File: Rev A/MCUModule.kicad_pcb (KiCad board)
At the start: 2 copper layers, 1 part, among them U1 RaspberryPi_Pico

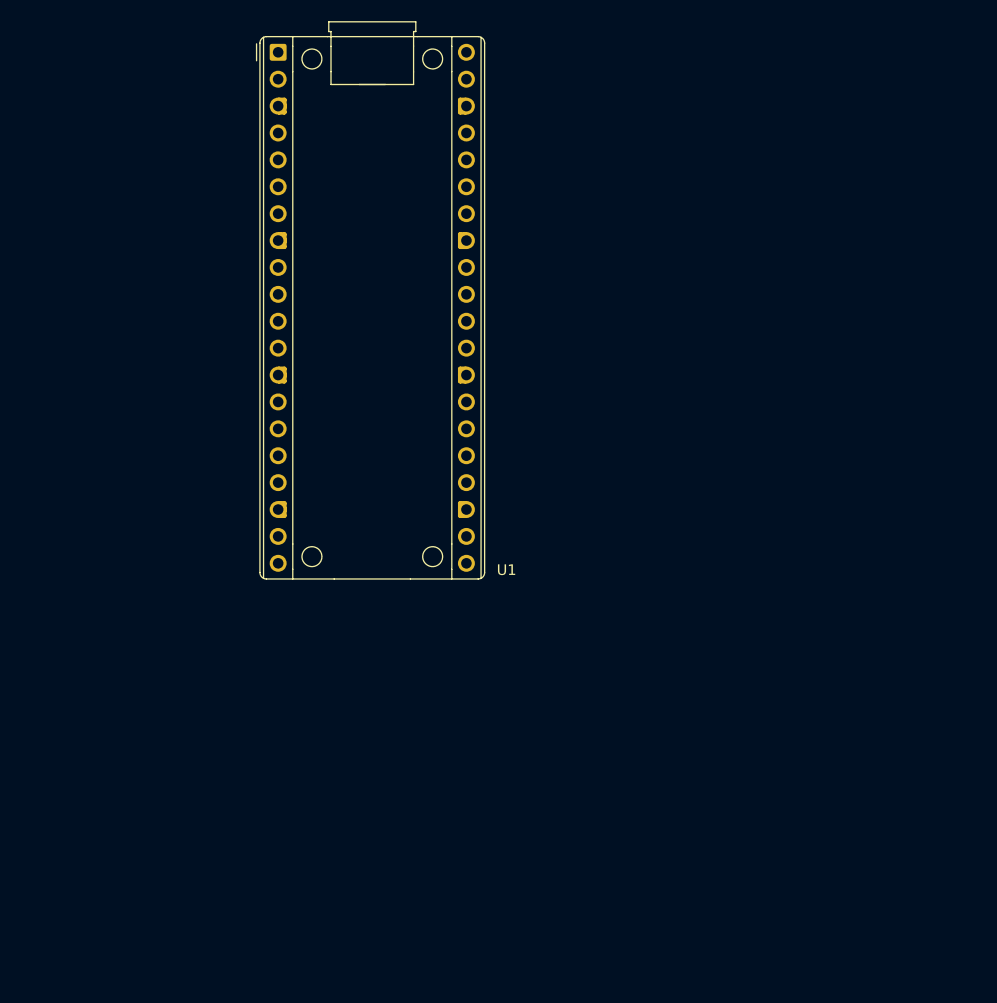
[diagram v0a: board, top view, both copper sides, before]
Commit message: routed
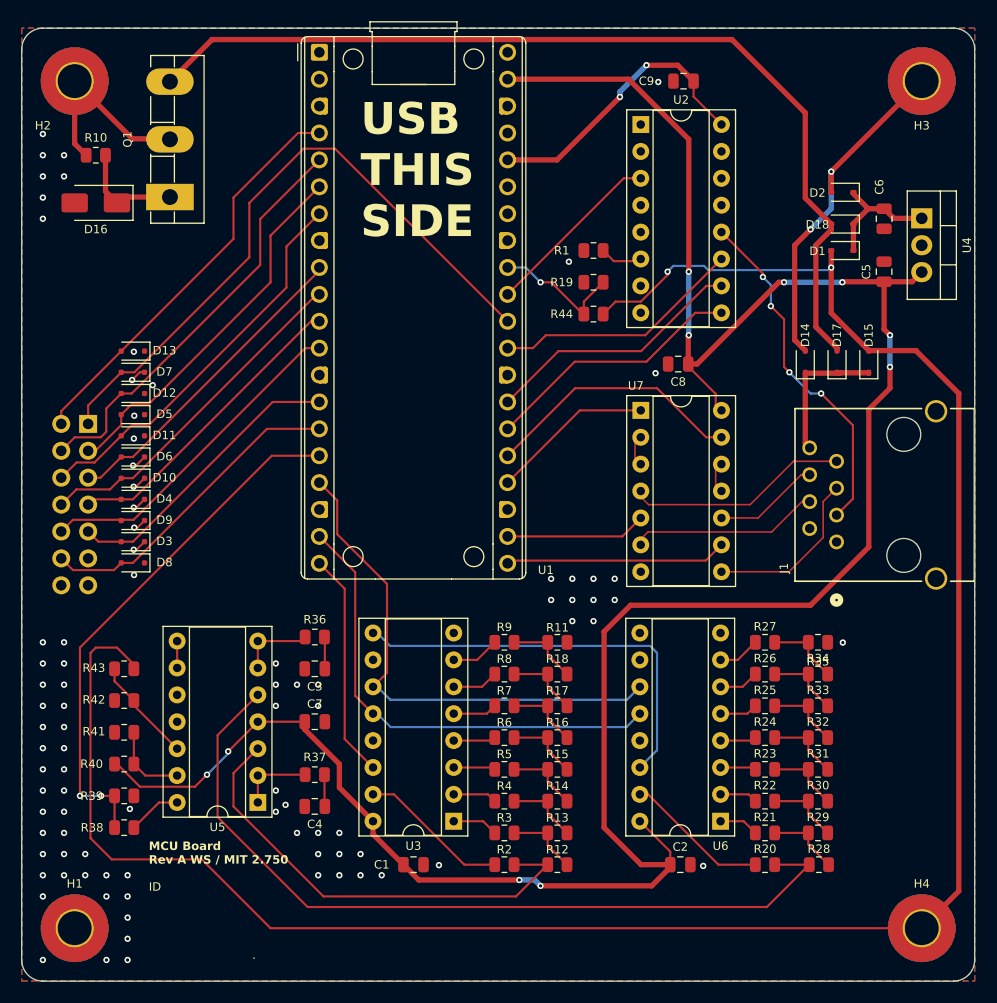
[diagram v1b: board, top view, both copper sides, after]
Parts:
- added C1: 0805,100nF,50V,X7R, Capacitor_SMD:C_0805_2012Metric, F.Cu at (134.0, 151.0)
- added C2: 0805,100nF,50V,X7R, Capacitor_SMD:C_0805_2012Metric, F.Cu at (159.2, 151.0)
- added C3: 0805,1uF,50V,X7R, Capacitor_SMD:C_0805_2012Metric, F.Cu at (124.7, 132.5)
- added C4: 0805,1uF,50V,X7R, Capacitor_SMD:C_0805_2012Metric, F.Cu at (124.7, 145.5)
- added C5: 0805,1uF,50V,X7R, Capacitor_SMD:C_0805_2012Metric, F.Cu at (178.4, 95.0)
- added C6: 0805,1uF,50V,X7R, Capacitor_SMD:C_0805_2012Metric, F.Cu at (178.4, 90.0)
- added C7: 0805,100nF,50V,X7R, Capacitor_SMD:C_0805_2012Metric, F.Cu at (124.7, 137.5)
- added C8: 0805,100nF,50V,X7R, Capacitor_SMD:C_0805_2012Metric, F.Cu at (159.0, 103.7)
- added C9: 0805,100nF,50V,X7R, Capacitor_SMD:C_0805_2012Metric, F.Cu at (159.5, 77.0)
- added D1: 1N5819WS, Diode_SMD:D_SOD-323, F.Cu at (174.5, 93.0)
- added D10: PESD3V3L1BA,115, Diode_SMD:D_SOD-323F, F.Cu at (107.5, 114.5)
- added D11: PESD3V3L1BA,115, Diode_SMD:D_SOD-323F, F.Cu at (107.5, 110.5)
- added D12: PESD3V3L1BA,115, Diode_SMD:D_SOD-323F, F.Cu at (107.5, 106.5)
- added D13: PESD3V3L1BA,115, Diode_SMD:D_SOD-323F, F.Cu at (107.5, 102.5)
- added D14: 1N5819WS, Diode_SMD:D_SOD-323, F.Cu at (171.0, 103.5)
- added D15: 1N5819WS, Diode_SMD:D_SOD-323, F.Cu at (177.0, 103.5)
- added D16: SMAZ15Z-13-F, Diode_SMD:D_SMA, F.Cu at (104.0, 88.5)
- added D17: 1N5819WS, Diode_SMD:D_SOD-323, F.Cu at (174.0, 103.5)
- added D18: 1N5819WS, Diode_SMD:D_SOD-323, F.Cu at (174.5, 90.5)
- added D2: 1N5819WS, Diode_SMD:D_SOD-323, F.Cu at (174.5, 87.5)
- added D3: PESD3V3L1BA,115, Diode_SMD:D_SOD-323F, F.Cu at (107.5, 120.5)
- added D4: PESD3V3L1BA,115, Diode_SMD:D_SOD-323F, F.Cu at (107.5, 116.5)
- added D5: PESD3V3L1BA,115, Diode_SMD:D_SOD-323F, F.Cu at (107.5, 108.5)
- added D6: PESD3V3L1BA,115, Diode_SMD:D_SOD-323F, F.Cu at (107.5, 112.5)
- added D7: PESD3V3L1BA,115, Diode_SMD:D_SOD-323F, F.Cu at (107.5, 104.5)
- added D8: PESD3V3L1BA,115, Diode_SMD:D_SOD-323F, F.Cu at (107.5, 122.5)
- added D9: PESD3V3L1BA,115, Diode_SMD:D_SOD-323F, F.Cu at (107.5, 118.5)
- added H1: M3 Hole, MountingHole:MountingHole_3.2mm_M3_Pad_TopBottom, F.Cu at (102.0, 157.0)
- added H2: M3 Hole, MountingHole:MountingHole_3.2mm_M3_Pad_TopBottom, F.Cu at (102.0, 77.0)
- added H3: M3 Hole, MountingHole:MountingHole_3.2mm_M3_Pad_TopBottom, F.Cu at (182.0, 77.0)
- added H4: M3 Hole, MountingHole:MountingHole_3.2mm_M3_Pad_TopBottom, F.Cu at (182.0, 157.0)
- added J1: RJ45_Shielded, Connectors_SurgicalLighting:CONN_A-2014-2S-4-N-R_ASM, F.Cu at (174.0, 120.5)
- added J2: 2x7 P2.54mm, Connector_PinHeader_2.54mm:PinHeader_2x07_P2.54mm_Vertical, B.Cu at (103.3, 109.4)
- added Q1: 2SD1047, Package_TO_SOT_THT:TO-3PB-3_Vertical, F.Cu at (111.0, 88.0)
- added R1: 0805,0, Resistor_SMD:R_0805_2012Metric, F.Cu at (151.0, 93.0)
- added R10: 0805,10k, Resistor_SMD:R_0805_2012Metric, F.Cu at (104.0, 84.0)
- added R11: 0805,20k, Resistor_SMD:R_0805_2012Metric, F.Cu at (147.6, 130.0)
- added R12: 0805,10k, Resistor_SMD:R_0805_2012Metric, F.Cu at (147.6, 151.0)
- added R13: 0805,10k, Resistor_SMD:R_0805_2012Metric, F.Cu at (147.6, 148.0)
- added R14: 0805,10k, Resistor_SMD:R_0805_2012Metric, F.Cu at (147.6, 145.0)
- added R15: 0805,10k, Resistor_SMD:R_0805_2012Metric, F.Cu at (147.6, 142.0)
- added R16: 0805,10k, Resistor_SMD:R_0805_2012Metric, F.Cu at (147.6, 139.0)
- added R17: 0805,10k, Resistor_SMD:R_0805_2012Metric, F.Cu at (147.6, 136.0)
- added R18: 0805,10k, Resistor_SMD:R_0805_2012Metric, F.Cu at (147.6, 133.0)
- added R19: 0805,10k, Resistor_SMD:R_0805_2012Metric, F.Cu at (151.0, 96.0)
- added R2: 0805,20k, Resistor_SMD:R_0805_2012Metric, F.Cu at (142.6, 151.0)
- added R20: 0805,20k, Resistor_SMD:R_0805_2012Metric, F.Cu at (167.2, 151.0)
- added R21: 0805,20k, Resistor_SMD:R_0805_2012Metric, F.Cu at (167.2, 148.0)
- added R22: 0805,20k, Resistor_SMD:R_0805_2012Metric, F.Cu at (167.2, 145.0)
- added R23: 0805,20k, Resistor_SMD:R_0805_2012Metric, F.Cu at (167.2, 142.0)
- added R24: 0805,20k, Resistor_SMD:R_0805_2012Metric, F.Cu at (167.2, 139.0)
- added R25: 0805,20k, Resistor_SMD:R_0805_2012Metric, F.Cu at (167.2, 136.0)
- added R26: 0805,20k, Resistor_SMD:R_0805_2012Metric, F.Cu at (167.2, 133.0)
- added R27: 0805,20k, Resistor_SMD:R_0805_2012Metric, F.Cu at (167.2, 130.0)
- added R28: 0805,10k, Resistor_SMD:R_0805_2012Metric, F.Cu at (172.3, 151.0)
- added R29: 0805,10k, Resistor_SMD:R_0805_2012Metric, F.Cu at (172.2, 148.0)
- added R3: 0805,20k, Resistor_SMD:R_0805_2012Metric, F.Cu at (142.6, 148.0)
- added R30: 0805,10k, Resistor_SMD:R_0805_2012Metric, F.Cu at (172.2, 145.0)
- added R31: 0805,10k, Resistor_SMD:R_0805_2012Metric, F.Cu at (172.2, 142.0)
- added R32: 0805,10k, Resistor_SMD:R_0805_2012Metric, F.Cu at (172.2, 139.0)
- added R33: 0805,10k, Resistor_SMD:R_0805_2012Metric, F.Cu at (172.2, 136.0)
- added R34: 0805,10k, Resistor_SMD:R_0805_2012Metric, F.Cu at (172.2, 133.0)
- added R35: 0805,20k, Resistor_SMD:R_0805_2012Metric, F.Cu at (172.2, 130.0)
- added R36: 0805,1k, Resistor_SMD:R_0805_2012Metric, F.Cu at (124.7, 129.5)
- added R37: 0805,1k, Resistor_SMD:R_0805_2012Metric, F.Cu at (124.7, 142.5)
- added R38: 0805,4.7k, Resistor_SMD:R_0805_2012Metric, F.Cu at (106.7, 147.5)
- added R39: 0805,10k, Resistor_SMD:R_0805_2012Metric, F.Cu at (106.7, 144.5)
- added R4: 0805,20k, Resistor_SMD:R_0805_2012Metric, F.Cu at (142.6, 145.0)
- added R40: 0805,10k, Resistor_SMD:R_0805_2012Metric, F.Cu at (106.7, 141.5)
- added R41: 0805,10k, Resistor_SMD:R_0805_2012Metric, F.Cu at (106.7, 138.5)
- added R42: 0805,10k, Resistor_SMD:R_0805_2012Metric, F.Cu at (106.7, 135.5)
- added R43: 0805,27k, Resistor_SMD:R_0805_2012Metric, F.Cu at (106.7, 132.5)
- added R44: 0805,33k, Resistor_SMD:R_0805_2012Metric, F.Cu at (151.0, 99.0)
- added R5: 0805,20k, Resistor_SMD:R_0805_2012Metric, F.Cu at (142.6, 142.0)
- added R6: 0805,20k, Resistor_SMD:R_0805_2012Metric, F.Cu at (142.6, 139.0)
- added R7: 0805,20k, Resistor_SMD:R_0805_2012Metric, F.Cu at (142.6, 136.0)
- added R8: 0805,20k, Resistor_SMD:R_0805_2012Metric, F.Cu at (142.6, 133.0)
- added R9: 0805,20k, Resistor_SMD:R_0805_2012Metric, F.Cu at (142.6, 130.0)
- added U2: 74HC4051, Package_DIP:DIP-16_W7.62mm_Socket, F.Cu at (155.5, 81.1)
- added U3: 74HC595, Package_DIP:DIP-16_W7.62mm_Socket, F.Cu at (137.8, 146.9)
- added U4: LM7805_TO220, Package_TO_SOT_THT:TO-220-3_Vertical, F.Cu at (182.0, 90.0)
- added U5: LM324, Package_DIP:DIP-14_W7.62mm_Socket, F.Cu at (119.3, 145.1)
- added U6: 74HC595, Package_DIP:DIP-16_W7.62mm_Socket, F.Cu at (163.0, 146.9)
- added U7: 74HC14, Package_DIP:DIP-14_W7.62mm_Socket, F.Cu at (155.5, 108.1)
- moved U1 3.89 mm to (134.0, 98.4)
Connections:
- net Net-(U1-GND-Pad13) renamed GND
- U1 pad 10: unconnected-(U1-GPIO7-Pad10) -> /PWM_Lights1
- U1 pad 11: unconnected-(U1-GPIO8-Pad11) -> /BatChgEna1
- U1 pad 12: unconnected-(U1-GPIO9-Pad12) -> /PWM_Lights2
- U1 pad 14: unconnected-(U1-GPIO10-Pad14) -> /BatChgEna2
- U1 pad 15: unconnected-(U1-GPIO11-Pad15) -> /RelaySelectHighPreference
- U1 pad 16: unconnected-(U1-GPIO12-Pad16) -> /12V_Wall_Bad
- U1 pad 17: unconnected-(U1-GPIO13-Pad17) -> SRCLK_DAC
- U1 pad 19: unconnected-(U1-GPIO14-Pad19) -> RCLK_DAC
- U1 pad 20: unconnected-(U1-GPIO15-Pad20) -> /DATA_DAC
- U1 pad 21: unconnected-(U1-GPIO16-Pad21) -> /~{RCLK_DISPLAY}
- U1 pad 22: unconnected-(U1-GPIO17-Pad22) -> /OE_DISPLAY
- U1 pad 24: unconnected-(U1-GPIO18-Pad24) -> /DATA_DISPLAY
- U1 pad 25: unconnected-(U1-GPIO19-Pad25) -> /SRCLK_DISPLAY
- U1 pad 26: unconnected-(U1-GPIO20-Pad26) -> /S2
- U1 pad 27: unconnected-(U1-GPIO21-Pad27) -> /S1
- U1 pad 29: unconnected-(U1-GPIO22-Pad29) -> /S0
- U1 pad 30: unconnected-(U1-RUN-Pad30) -> /ModuleENA
- U1 pad 31: unconnected-(U1-GPIO26_ADC0-Pad31) -> /AnalogMuxOut
- U1 pad 32: unconnected-(U1-GPIO27_ADC1-Pad32) -> Net-(U1-GPIO27_ADC1)
- U1 pad 36: unconnected-(U1-3V3-Pad36) -> +3.3V
- U1 pad 39: unconnected-(U1-VSYS-Pad39) -> +5V
- U1 pad 4: unconnected-(U1-GPIO2-Pad4) -> /DisableBackupPico
- U1 pad 5: unconnected-(U1-GPIO3-Pad5) -> /PowerModuleEna1
- U1 pad 6: unconnected-(U1-GPIO4-Pad6) -> /BoostEna1
- U1 pad 7: unconnected-(U1-GPIO5-Pad7) -> /PowerModuleEna2
- U1 pad 9: unconnected-(U1-GPIO6-Pad9) -> /BoostEna2
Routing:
- net +5V: track 0.00 -> 223.7 mm, vias 0 -> 10
- net /12V_Wall: track 0.00 -> 201.8 mm, vias 0 -> 2
- net /15V_SOLAR: track 0.00 -> 89.4 mm
- net /Shift Register Based DAC 1/AnalogOut_Unbuffered: track 0.00 -> 77.4 mm
- net /ModuleENA: track 0.00 -> 61.2 mm
- net /12V_Wall_Bad: track 0.00 -> 50.4 mm, vias 0 -> 2
- net SRCLK_DAC: track 0.00 -> 48.3 mm
- net RCLK_DAC: track 0.00 -> 44.7 mm
- net /Shift Register Based DAC 0/AnalogOut_Unbuffered: track 0.00 -> 44.0 mm
- net /PowerModuleEna1: track 0.00 -> 39.6 mm
- net /DisableBackupPico: track 0.00 -> 38.7 mm
- net /Shift Register Based DAC 0/DataOut: track 0.00 -> 38.7 mm
- net /PowerModuleEna2: track 0.00 -> 37.0 mm
- net /BoostEna1: track 0.00 -> 35.3 mm
- net /DIM: track 0.00 -> 33.1 mm, vias 0 -> 4
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- added copper zone on B.Cu, net GND
- added copper zone on F.Cu, net GND
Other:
- board outline added: 90 x 90 mm
- board text added: "ID ."
- board text added: "MCU Board Rev A WS / MIT 2.750"
- board text added: "USB THIS SIDE"
